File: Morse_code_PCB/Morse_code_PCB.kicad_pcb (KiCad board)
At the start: 2 copper layers, 60 parts, among them J1 USB_C_Receptacle_USB2.0, J2 INPUT, J3 OUTPUT, J4 Conn_01x02_Female, Q1 AO3400A, Q2 AO3401A, Q3 AO3400A, Q4 AO3401A, SW1 RotaryEncoder_Switch, U1 STM32F030F4Px, U2 OLED_12864, U3 MCP73831-2-OT, U4 CH340E, U5 LP5907MFX-3.3, U6 24AA02-OT

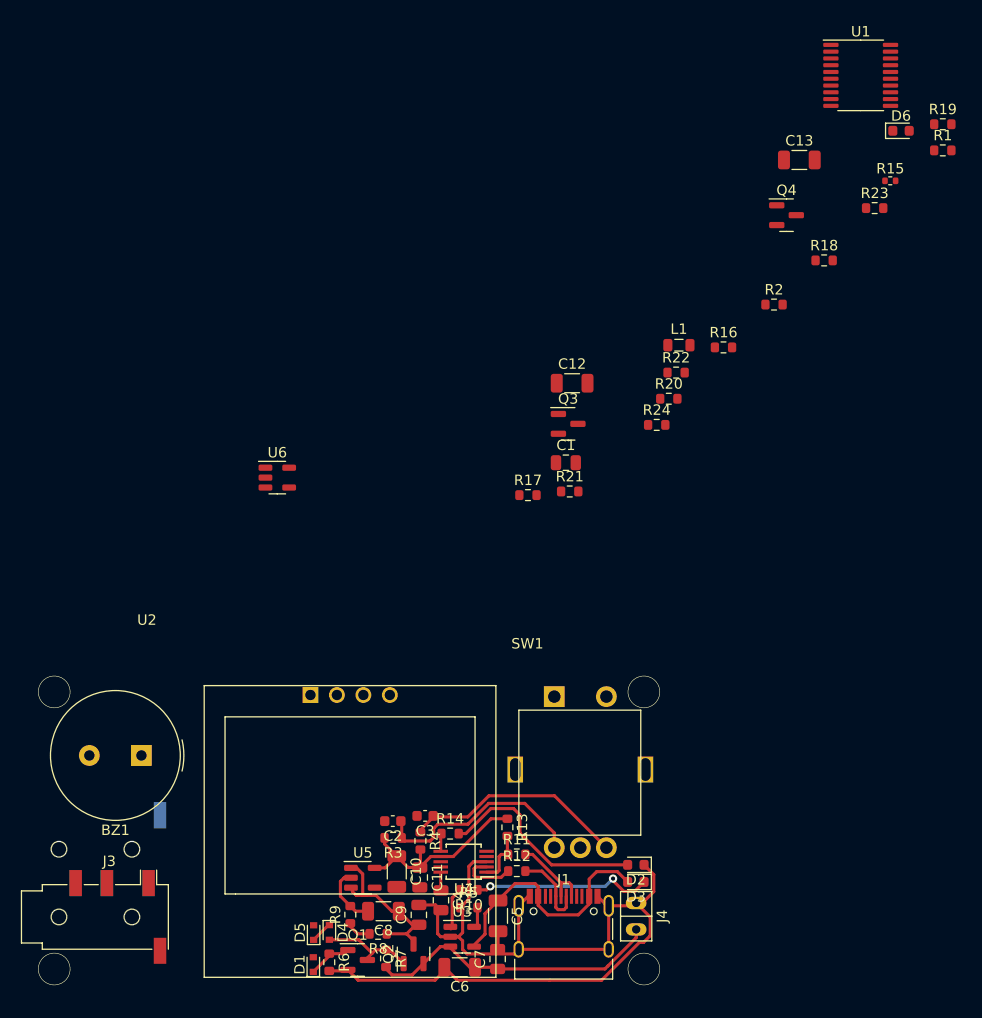
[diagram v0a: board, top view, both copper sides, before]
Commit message: PCB画完 Signed-off-by: kevin <kevin@lmve.net>
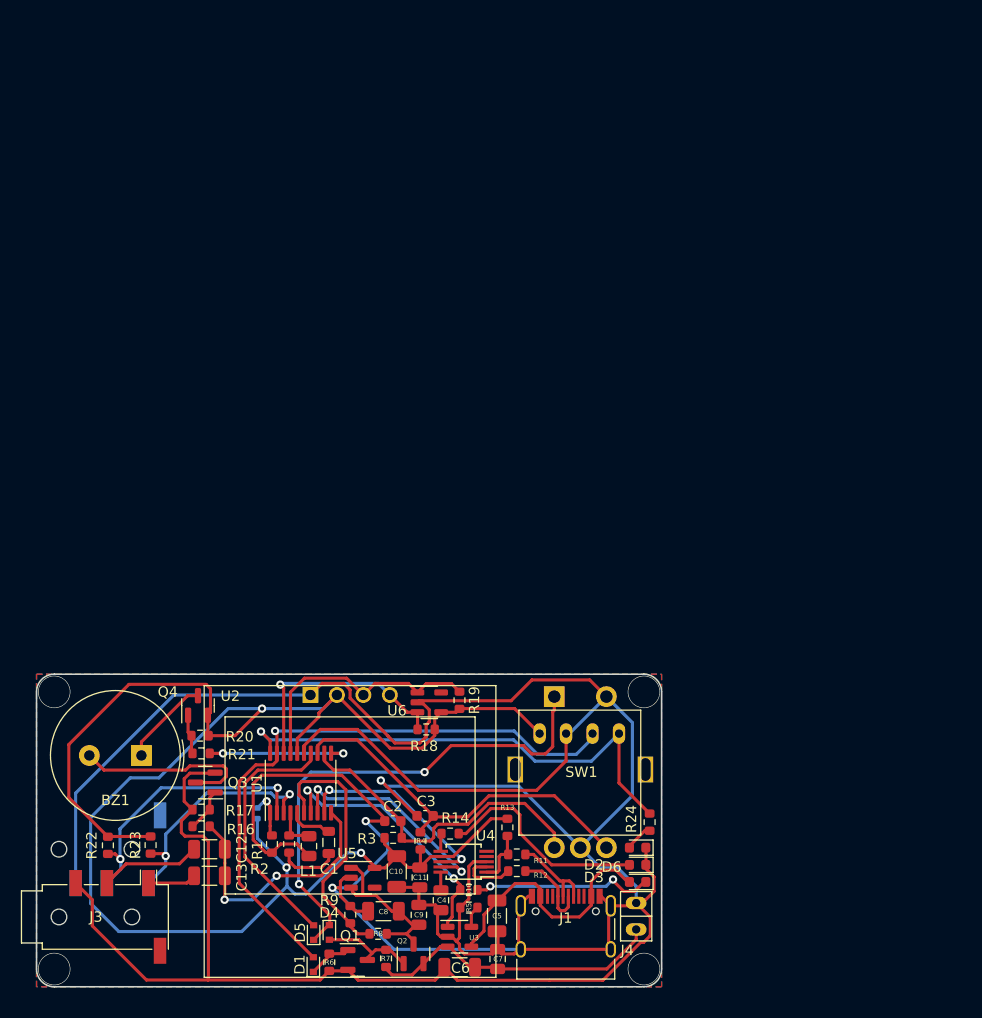
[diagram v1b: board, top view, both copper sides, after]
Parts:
- added J5: Conn_01x04_Female, MY:SIP-4, B.Cu at (122.1, 137.7)
- R15: moved to B.Cu
- moved R1 92.6 mm to (92.6, 148.3), turned to 90 degrees
- moved R23 92.6 mm to (81.0, 148.4), turned to -90 degrees
- moved C13 89.0 mm to (86.6, 151.3)
- moved U1 86.6 mm to (95.3, 142.4), turned to 90 degrees
- moved R15 85.9 mm to (91.2, 145.3), turned to 90 degrees
- moved Q4 73.5 mm to (85.5, 135.0), turned to 90 degrees
- moved D6 73.3 mm to (127.7, 148.7), turned to 180 degrees
- moved R19 72.2 mm to (110.6, 134.5), turned to -90 degrees
- moved R22 70.9 mm to (76.8, 148.4), turned to -90 degrees
- moved R2 69.6 mm to (94.2, 148.3), turned to -90 degrees
- moved R16 68.0 mm to (85.8, 146.6)
- moved R18 59.0 mm to (107.4, 137.3)
- moved L1 58.4 mm to (98.0, 148.2), turned to 90 degrees
- moved C12 56.7 mm to (86.6, 148.8)
- moved R20 55.4 mm to (85.7, 137.9)
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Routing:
- net GND: track 97.3 -> 384.1 mm, vias 0 -> 3
- net VCC: track 19.6 -> 177.0 mm, vias 0 -> 3
- net PWR_EN: track 0.00 -> 59.7 mm, vias 0 -> 1
- net RUN_LED: track 0.00 -> 48.0 mm, vias 0 -> 1
- net K1: track 2.09 -> 48.3 mm, vias 0 -> 2
- net TICK_A: track 0.00 -> 26.4 mm, vias 0 -> 2
- net PWM: track 0.00 -> 25.1 mm, vias 0 -> 2
- net IIC_SCL: track 0.00 -> 24.8 mm
- net K1_DET: track 0.00 -> 24.3 mm
- net TICK_B: track 0.00 -> 22.8 mm, vias 0 -> 2
- net IIC_SDL: track 0.00 -> 22.7 mm, vias 0 -> 1
- net BAT_ADC: track 2.44 -> 25.2 mm
- net RXD: track 0.00 -> 21.5 mm, vias 0 -> 2
- net BAT_CHG_DET: track 4.13 -> 25.2 mm, vias 0 -> 2
- net TXD: track 0.00 -> 20.0 mm, vias 0 -> 2
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- added copper zone on B.Cu, net GND
- added copper zone on F.Cu, net GND
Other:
- board outline added: 60 x 30 mm
- board text added: "4.7V +"
- board text added: "BOOT_0 PUTUP"
- board text added: "X X G V"
